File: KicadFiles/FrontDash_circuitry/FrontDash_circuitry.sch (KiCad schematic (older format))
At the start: 32 parts, among them J1 ICSP, J2 Conn_01x02_Male, J3 Conn_01x02_Male, SW1 SW_Push, U1 ATmega328P-AU, U2 DS3231M, U3 MCP2515-EST, U4 MCP2551-I-P, Y1 10MHz, Y1 Crystal

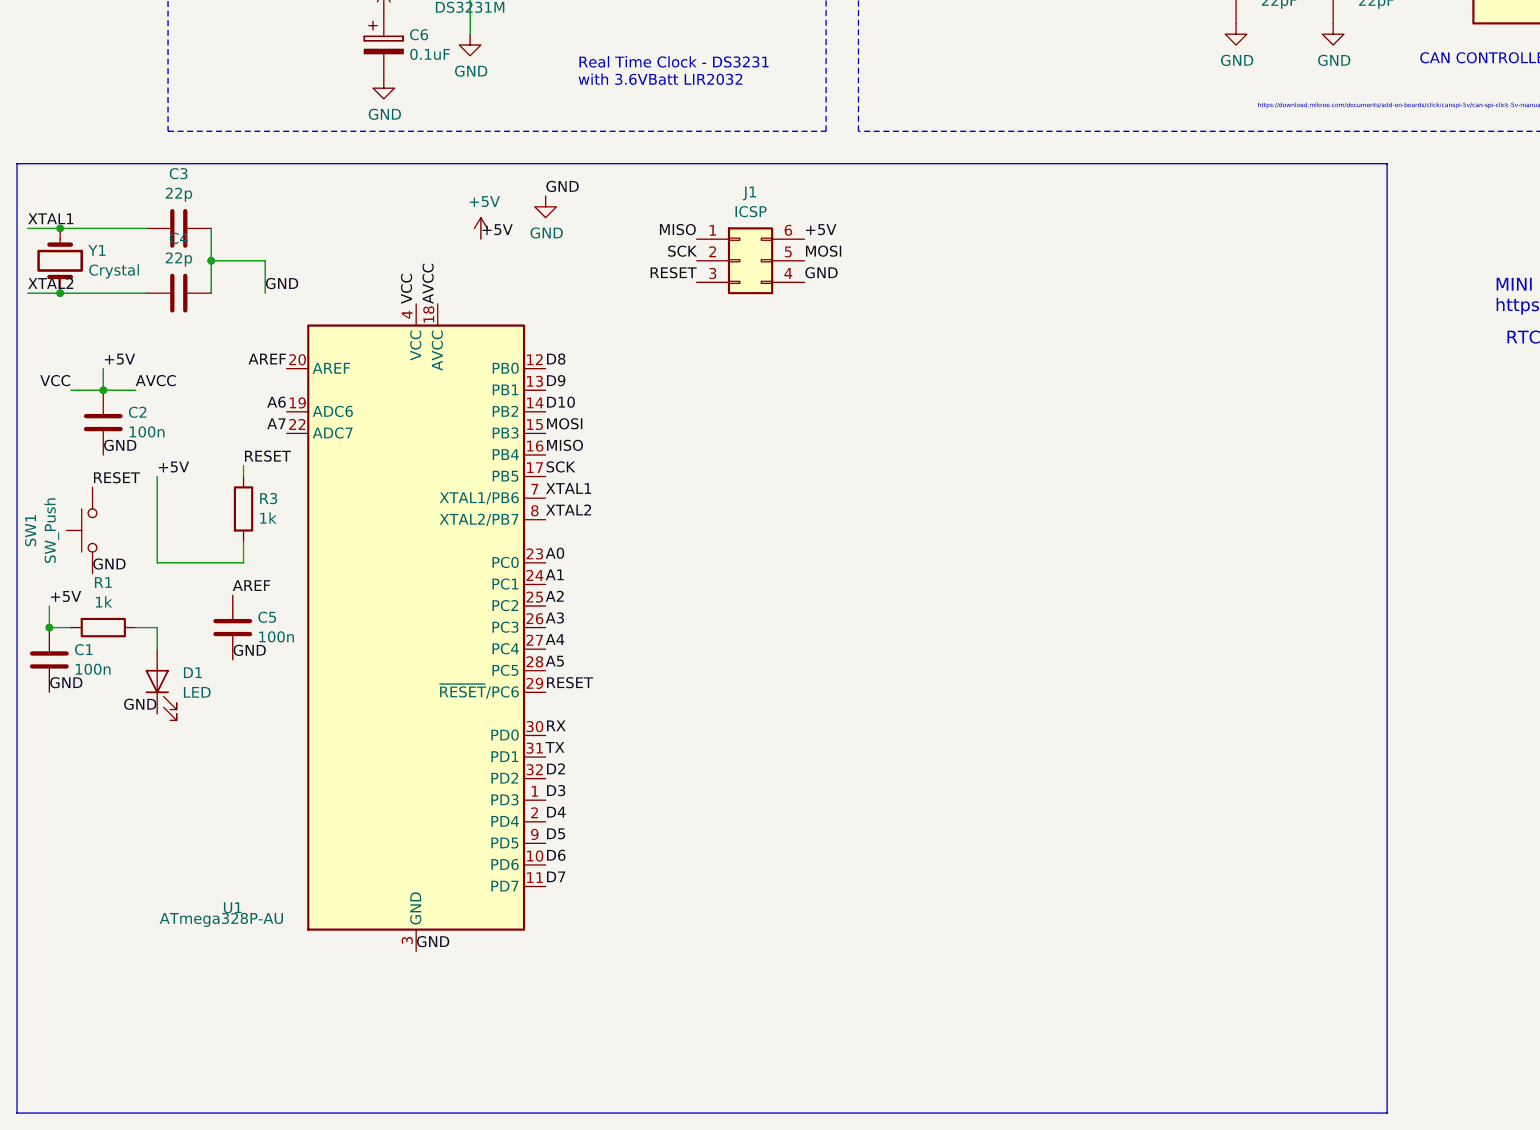
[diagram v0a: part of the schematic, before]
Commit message: nano completed
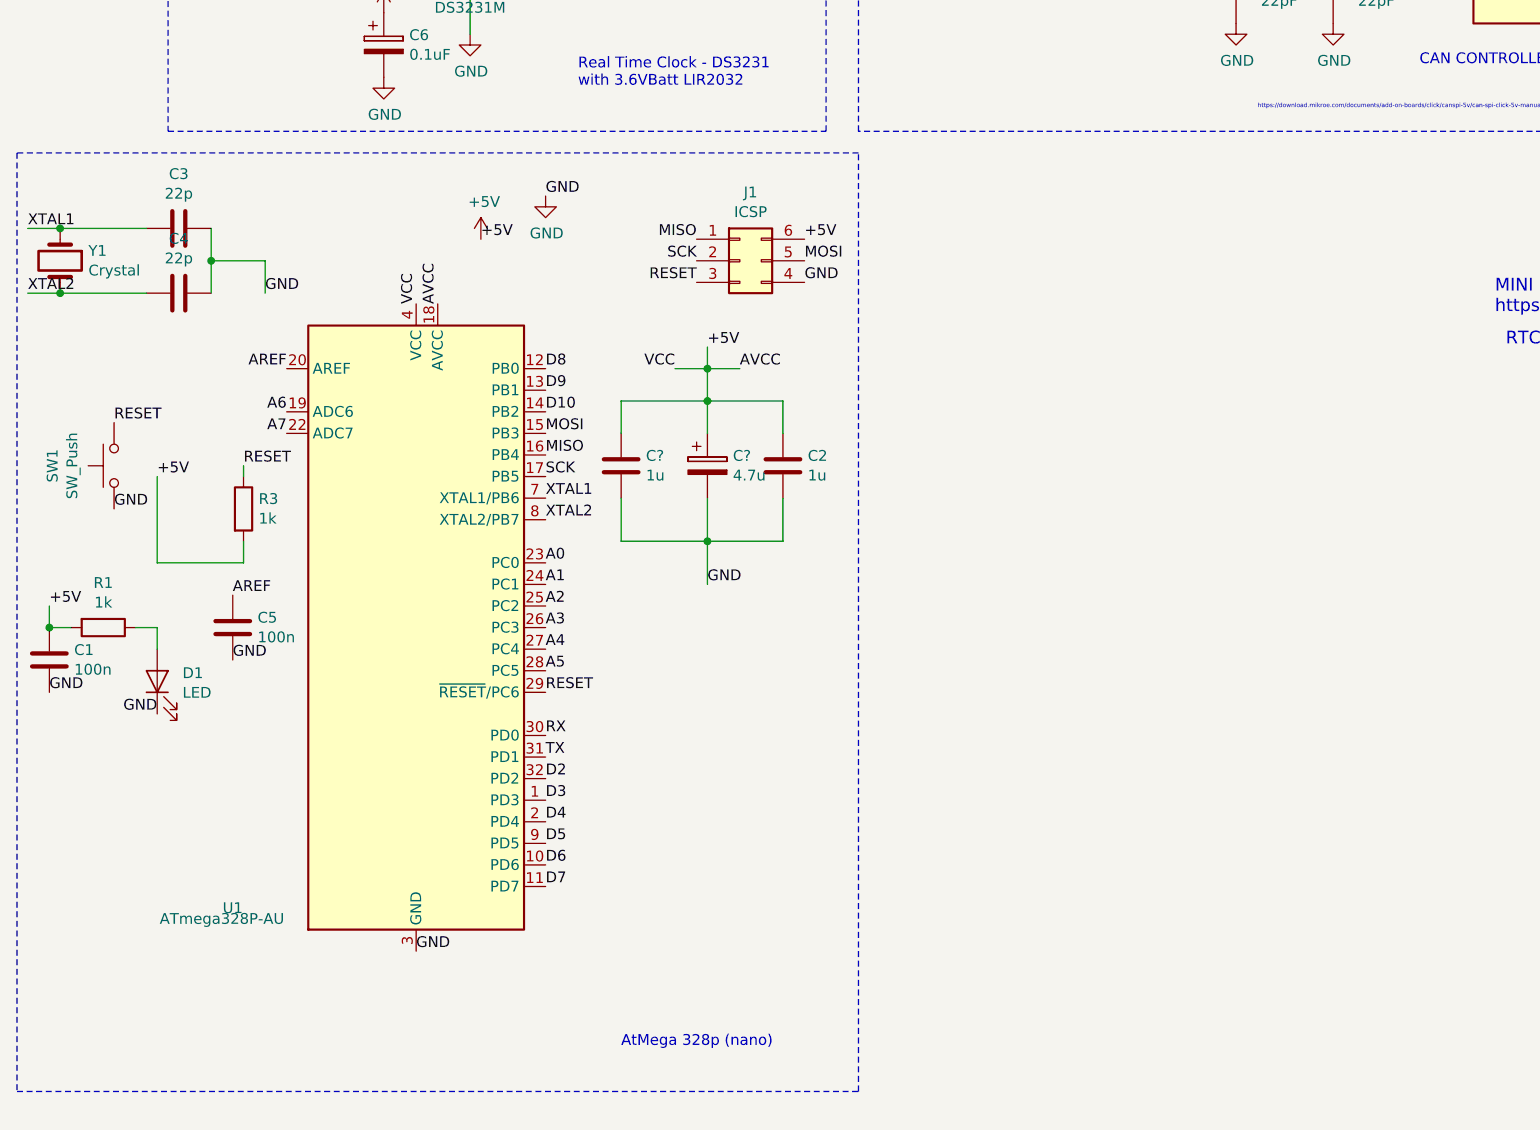
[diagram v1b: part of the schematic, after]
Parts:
- added C?: 1u, symbol Device:C
- added C?: 4.7u, symbol Device:CP
- C2: value 100n -> 1u
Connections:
- net +5V: now also C?.1, C?.1
- net GND: now also C?.2, C?.2
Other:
- note added: "AtMega 328p (nano)\n"
- moved on the sheet: C2, SW1
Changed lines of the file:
@@
 EESchema Schematic File Version 4
 LIBS:FrontDash_circuitry-cache
-EELAYER 26 0
+EELAYER 28 0
 EELAYER END
 $Descr A4 11693 8268
@@
 Wire Wire Line
 	1450 3800 1450 3950
-Wire Bus Line
-	550  7750 6900 7750
-Wire Bus Line
-	6900 3350 550  3350
-Wire Bus Line
-	550  3350 550  7750
-Wire Bus Line
-	6900 3350 6900 7750
 Text Label 2400 4000 1    50   ~ 0
 VCC
@@
 AVCC
 Wire Wire Line
-	800  4400 950  4400
-Text Label 1100 4400 0    50   ~ 0
+	3600 4300 3750 4300
+Text Label 3900 4300 0    50   ~ 0
 AVCC
-Text Label 800  4400 2    50   ~ 0
+Text Label 3600 4300 2    50   ~ 0
 VCC
 $Comp
 L Device:C C2
 U 1 1 5BEEEC4C
-P 950 4550
-F 0 "C2" H 1065 4596 50  0000 L CNN
-F 1 "100n" H 1065 4505 50  0000 L CNN
-F 2 "" H 988 4400 50  0001 C CNN
-F 3 "~" H 950 4550 50  0001 C CNN
-	1    950  4550
+P 4100 4750
+F 0 "C2" H 4215 4796 50  0000 L CNN
+F 1 "1u" H 4215 4705 50  0000 L CNN
+F 2 "" H 4138 4600 50  0001 C CNN
+F 3 "~" H 4100 4750 50  0001 C CNN
+	1    4100 4750
 	1    0    0    -1
 $EndComp
@@
 	1    0    0    -1
 $EndComp
-Connection ~ 950  4400
-Wire Wire Line
-	950  4300 950  4400
-Wire Wire Line
-	1100 4400 950  4400
+Connection ~ 3750 4300
+Wire Wire Line
+	3750 4200 3750 4300
+Wire Wire Line
+	3900 4300 3750 4300
 Text Label 3000 5800 0    50   ~ 0
 RESET
@@
 L Switch:SW_Push SW1
 U 1 1 5BF1B5B4
-P 900 5050
-F 0 "SW1" H 900 5335 50  0000 C CNN
-F 1 "SW_Push" H 900 5244 50  0000 C CNN
-F 2 "" H 900 5250 50  0001 C CNN
-F 3 "" H 900 5250 50  0001 C CNN
-	1    900  5050
+P 1000 4750
+F 0 "SW1" H 1000 5035 50  0000 C CNN
+F 1 "SW_Push" H 1000 4944 50  0000 C CNN
+F 2 "" H 1000 4950 50  0001 C CNN
+F 3 "" H 1000 4950 50  0001 C CNN
+	1    1000 4750
 	0    -1   -1   0
 $EndComp
@@
 Wire Wire Line
 	1600 5200 1200 5200
-Text Label 950  4700 0    50   ~ 0
+Text Label 3750 5300 0    50   ~ 0
 GND
 Text Label 2400 7000 0    50   ~ 0
@@
 	1    0    0    -1
 $EndComp
-Text Label 900  4850 0    50   ~ 0
+Text Label 1000 4550 0    50   ~ 0
 RESET
-Text Label 900  5250 0    50   ~ 0
+Text Label 1000 4950 0    50   ~ 0
 GND
 Text Label 1200 4800 0    50   ~ 0
@@
 Text Label 3700 3800 2    50   ~ 0
 SCK
-Text Label 950  4300 0    50   ~ 0
+Text Label 3750 4200 0    50   ~ 0
 +5V
 Text Label 700  5400 0    50   ~ 0
@@
 Text Notes 7450 4200 0    59   ~ 0
 RTC
+$Comp
+L Device:C C?
+U 1 1 5C01A2F6
+P 3350 4750
+F 0 "C?" H 3465 4796 50  0000 L CNN
+F 1 "1u" H 3465 4705 50  0000 L CNN
+F 2 "" H 3388 4600 50  0001 C CNN
+F 3 "~" H 3350 4750 50  0001 C CNN
+	1    3350 4750
+	1    0    0    -1
+$EndComp
+$Comp
+L Device:CP C?
+U 1 1 5C023C80
+P 3750 4750
+F 0 "C?" H 3868 4796 50  0000 L CNN
+F 1 "4.7u" H 3868 4705 50  0000 L CNN
+F 2 "" H 3788 4600 50  0001 C CNN
+F 3 "~" H 3750 4750 50  0001 C CNN
+	1    3750 4750
+	1    0    0    -1
+$EndComp
+Wire Wire Line
+	3750 4300 3750 4450
+Wire Wire Line
+	3350 4600 3350 4450
+Wire Wire Line
+	3350 4450 3750 4450
+Connection ~ 3750 4450
+Wire Wire Line
+	3750 4450 3750 4600
+Wire Wire Line
+	3750 4450 4100 4450
+Wire Wire Line
+	4100 4450 4100 4600
+Wire Wire Line
+	4100 4900 4100 5100
+Wire Wire Line
+	4100 5100 3750 5100
+Wire Wire Line
+	3350 5100 3350 4900
+Wire Wire Line
+	3750 4900 3750 5100
+Connection ~ 3750 5100
+Wire Wire Line
+	3750 5100 3350 5100
+Wire Wire Line
+	3750 5100 3750 5300
+Text Notes 3350 7450 0    50   ~ 0
+AtMega 328p (nano)\n
+Wire Notes Line
+	550  7650 4450 7650
+Wire Notes Line
+	4450 7650 4450 3300
+Wire Notes Line
+	4450 3300 550  3300
+Wire Notes Line
+	550  3300 550  7650
 $EndSCHEMATC

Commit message: Front dash mini sd card is almost done
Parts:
- added C? (x2): 100 nF, symbol Device:C
- added J?: Micro_SD_Card, symbol Connector:Micro_SD_Card
- added U?: LP2985-3.3, Package_TO_SOT_SMD:SOT-23-5, symbol Regulator_Linear:LP2985-3.3
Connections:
- net labels added: CD_SD, CLK
- wire segments 83 -> 99
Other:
- note added: "Linear Regulator"
- note added: "https://learn.adafruit.com/assets/35635"
- note added: "insert CD54HC4050 here (level shifter)"
- note removed: "RTC"
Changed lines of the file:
@@
 EESchema Schematic File Version 4
 LIBS:FrontDash_circuitry-cache
-EELAYER 28 0
+EELAYER 26 0
 EELAYER END
 $Descr A4 11693 8268
@@
 Text Notes 7400 4050 0    59   ~ 0
 MINI SD CARD \nhttps://learn.adafruit.com/adafruit-micro-sd-breakout-board-card-tutorial/download
-Text Notes 7450 4200 0    59   ~ 0
-RTC
 $Comp
 L Device:C C?
@@
 Wire Notes Line
 	550  3300 550  7650
+$Comp
+L Regulator_Linear:LP2985-3.3 U?
+U 1 1 5C075051
+P 6050 3900
+F 0 "U?" H 6050 4242 50  0000 C CNN
+F 1 "LP2985-3.3" H 6050 4151 50  0000 C CNN
+F 2 "Package_TO_SOT_SMD:SOT-23-5" H 6050 4225 50  0001 C CNN
+F 3 "http://www.ti.com/lit/ds/symlink/lp2985.pdf" H 6050 3900 50  0001 C CNN
+	1    6050 3900
+	1    0    0    -1
+$EndComp
+$Comp
+L power:+3V3 #PWR?
+U 1 1 5C0753B8
+P 6550 3750
+F 0 "#PWR?" H 6550 3600 50  0001 C CNN
+F 1 "+3V3" H 6565 3923 50  0000 C CNN
+F 2 "" H 6550 3750 50  0001 C CNN
+F 3 "" H 6550 3750 50  0001 C CNN
+	1    6550 3750
+	1    0    0    -1
+$EndComp
+Wire Wire Line
+	6450 3800 6550 3800
+Wire Wire Line
+	6550 3800 6550 3750
+$Comp
+L power:GND #PWR?
+U 1 1 5C0774A6
+P 6050 4200
+F 0 "#PWR?" H 6050 3950 50  0001 C CNN
+F 1 "GND" H 6055 4027 50  0000 C CNN
+F 2 "" H 6050 4200 50  0001 C CNN
+F 3 "" H 6050 4200 50  0001 C CNN
+	1    6050 4200
+	1    0    0    -1
+$EndComp
+$Comp
+L power:+5V #PWR?
+U 1 1 5C0779E3
+P 5550 3800
+F 0 "#PWR?" H 5550 3650 50  0001 C CNN
+F 1 "+5V" H 5565 3973 50  0000 C CNN
+F 2 "" H 5550 3800 50  0001 C CNN
+F 3 "" H 5550 3800 50  0001 C CNN
+	1    5550 3800
+	1    0    0    -1
+$EndComp
+Wire Wire Line
+	5650 3800 5550 3800
+$Comp
+L Device:C C?
+U 1 1 5C079EC3
+P 6800 3950
+F 0 "C?" H 6915 3996 50  0000 L CNN
+F 1 "100 nF" H 6915 3905 50  0000 L CNN
+F 2 "" H 6838 3800 50  0001 C CNN
+F 3 "~" H 6800 3950 50  0001 C CNN
+	1    6800 3950
+	1    0    0    -1
+$EndComp
+$Comp
+L Device:C C?
+U 1 1 5C07A03B
+P 5100 3950
+F 0 "C?" H 5215 3996 50  0000 L CNN
+F 1 "100 nF" H 5215 3905 50  0000 L CNN
+F 2 "" H 5138 3800 50  0001 C CNN
+F 3 "~" H 5100 3950 50  0001 C CNN
+	1    5100 3950
+	1    0    0    -1
+$EndComp
+Wire Wire Line
+	5550 3800 5500 3800
+Connection ~ 5550 3800
+Wire Wire Line
+	6550 3800 6800 3800
+Connection ~ 6550 3800
+$Comp
+L power:GND #PWR?
+U 1 1 5C07E085
+P 5100 4100
+F 0 "#PWR?" H 5100 3850 50  0001 C CNN
+F 1 "GND" H 5105 3927 50  0000 C CNN
+F 2 "" H 5100 4100 50  0001 C CNN
+F 3 "" H 5100 4100 50  0001 C CNN
+	1    5100 4100
+	1    0    0    -1
+$EndComp
+$Comp
+L power:GND #PWR?
+U 1 1 5C07E0DA
+P 6800 4100
+F 0 "#PWR?" H 6800 3850 50  0001 C CNN
+F 1 "GND" H 6805 3927 50  0000 C CNN
+F 2 "" H 6800 4100 50  0001 C CNN
+F 3 "" H 6800 4100 50  0001 C CNN
+	1    6800 4100
+	1    0    0    -1
+$EndComp
+Wire Wire Line
+	5650 3900 5500 3900
+Wire Wire Line
+	5500 3900 5500 3800
+Connection ~ 5500 3800
+Wire Wire Line
+	5500 3800 5100 3800
+Text Notes 5250 3550 0    50   ~ 0
+Linear Regulator
+Wire Notes Line
+	4600 3300 11050 3300
+Wire Notes Line
+	11050 3300 11050 6450
+Wire Notes Line
+	11050 6450 4600 6450
+Wire Notes Line
+	4600 6450 4600 3300
+Text Notes 5700 5650 0    50   ~ 0
+insert CD54HC4050 here (level shifter)
+$Comp
+L Connector:Micro_SD_Card J?
+U 1 1 5C085268
+P 8600 5450
+F 0 "J?" H 8550 6167 50  0000 C CNN
+F 1 "Micro_SD_Card" H 8550 6076 50  0000 C CNN
+F 2 "" H 9750 5750 50  0001 C CNN
+F 3 "http://katalog.we-online.de/em/datasheet/693072010801.pdf" H 8600 5450 50  0001 C CNN
+	1    8600 5450
+	1    0    0    -1
+$EndComp
+$Comp
+L power:GND #PWR?
+U 1 1 5C0855B0
+P 9400 6050
+F 0 "#PWR?" H 9400 5800 50  0001 C CNN
+F 1 "GND" H 9405 5877 50  0000 C CNN
+F 2 "" H 9400 6050 50  0001 C CNN
+F 3 "" H 9400 6050 50  0001 C CNN
+	1    9400 6050
+	1    0    0    -1
+$EndComp
+Wire Wire Line
+	7700 5650 7550 5650
+Wire Wire Line
+	7700 5550 7300 5550
+Wire Wire Line
+	7300 5450 7700 5450
+Wire Wire Line
+	7700 5350 7300 5350
+Wire Wire Line
+	7300 5250 7700 5250
+Wire Wire Line
+	7700 5150 7300 5150
+Wire Wire Line
+	7300 5750 7700 5750
+Wire Wire Line
+	7300 5850 7700 5850
+$Comp
+L power:GND #PWR?
+U 1 1 5C0B5CF7
+P 7550 5650
+F 0 "#PWR?" H 7550 5400 50  0001 C CNN
+F 1 "GND" H 7555 5477 50  0000 C CNN
+F 2 "" H 7550 5650 50  0001 C CNN
+F 3 "" H 7550 5650 50  0001 C CNN
+	1    7550 5650
+	0    1    1    0
+$EndComp
+$Comp
+L power:+3V3 #PWR?
+U 1 1 5C0B5E0C
+P 7300 5450
+F 0 "#PWR?" H 7300 5300 50  0001 C CNN
+F 1 "+3V3" H 7315 5623 50  0000 C CNN
+F 2 "" H 7300 5450 50  0001 C CNN
+F 3 "" H 7300 5450 50  0001 C CNN
+	1    7300 5450
+	0    -1   -1   0
+$EndComp
+Text Label 7300 5550 0    50   ~ 0
+CLK
+Text Label 7300 5250 0    50   ~ 0
+CD_SD
+Text Notes 6050 4950 0    50   ~ 0
+https://learn.adafruit.com/assets/35635
 $EndSCHEMATC
